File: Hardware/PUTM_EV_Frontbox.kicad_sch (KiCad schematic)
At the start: 4 parts

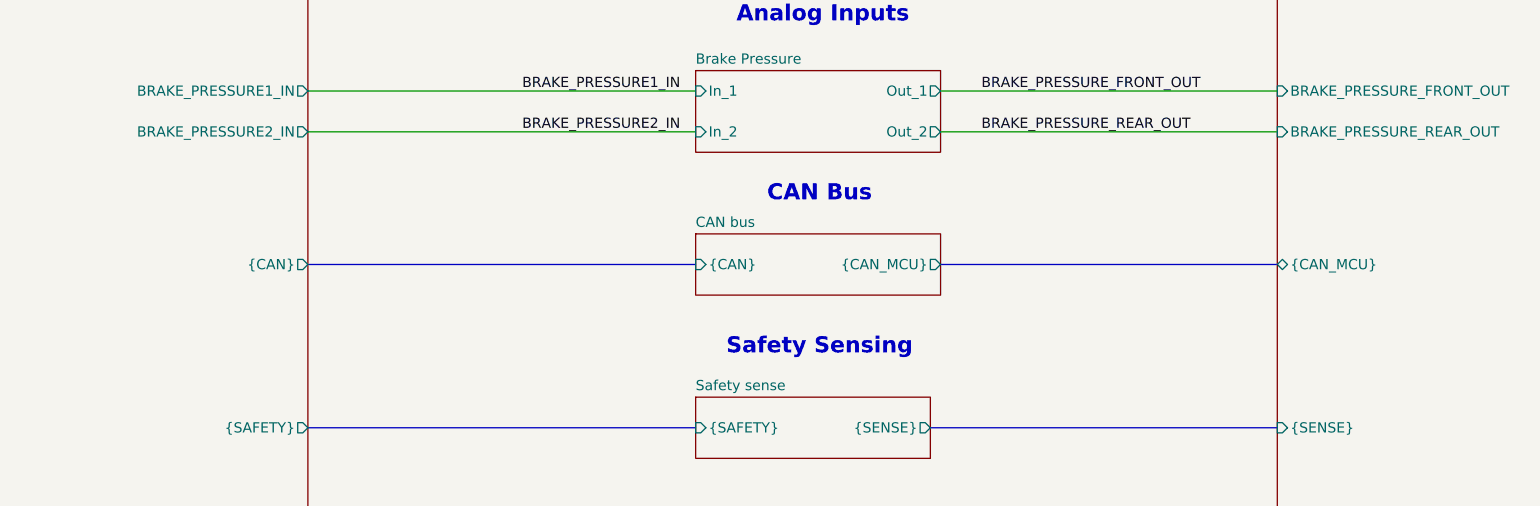
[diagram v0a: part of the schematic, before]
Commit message: Changes in CAN section
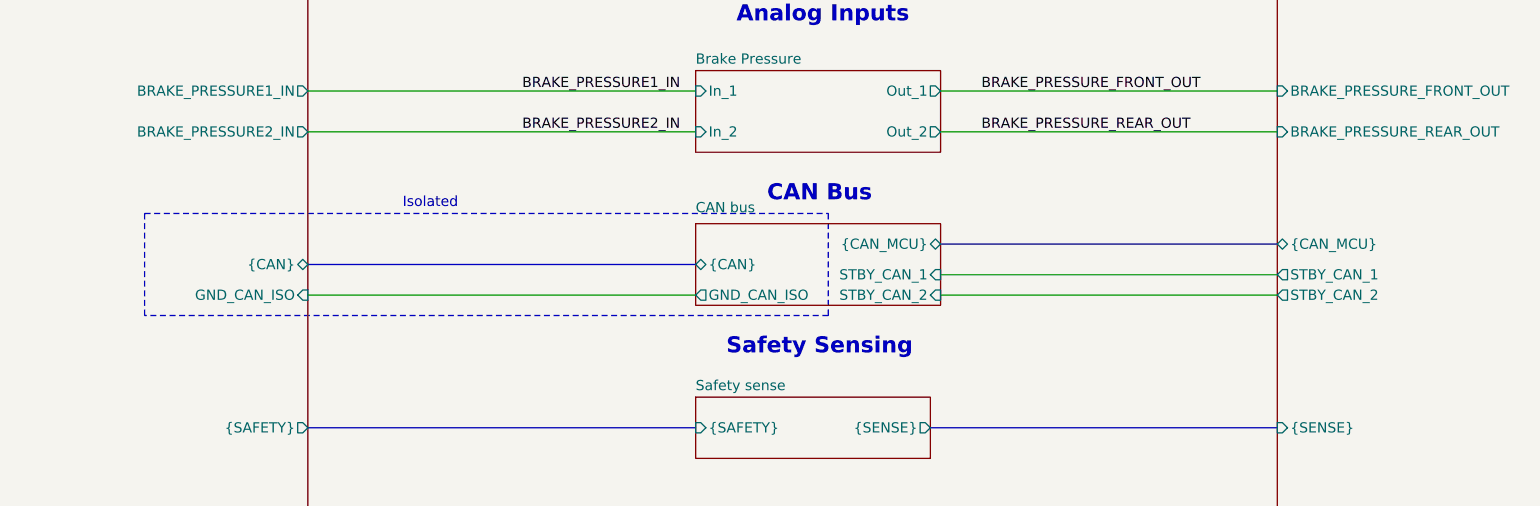
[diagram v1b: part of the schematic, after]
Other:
- sheet CAN bus ports: added GND_CAN_ISO, STBY_CAN_1, STBY_CAN_2; removed none
- sheet Connector ports: added GND_CAN_ISO; removed none
- sheet MCU ports: added STBY_CAN_1, STBY_CAN_2; removed none
- note added: "Isolated"
